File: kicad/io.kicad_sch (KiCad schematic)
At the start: 11 parts, among them J2 UART, P1 Mini-DIN_6pins_ver3, U13 uSD adapter, U14 8259, U16 16550, U17 T6963C

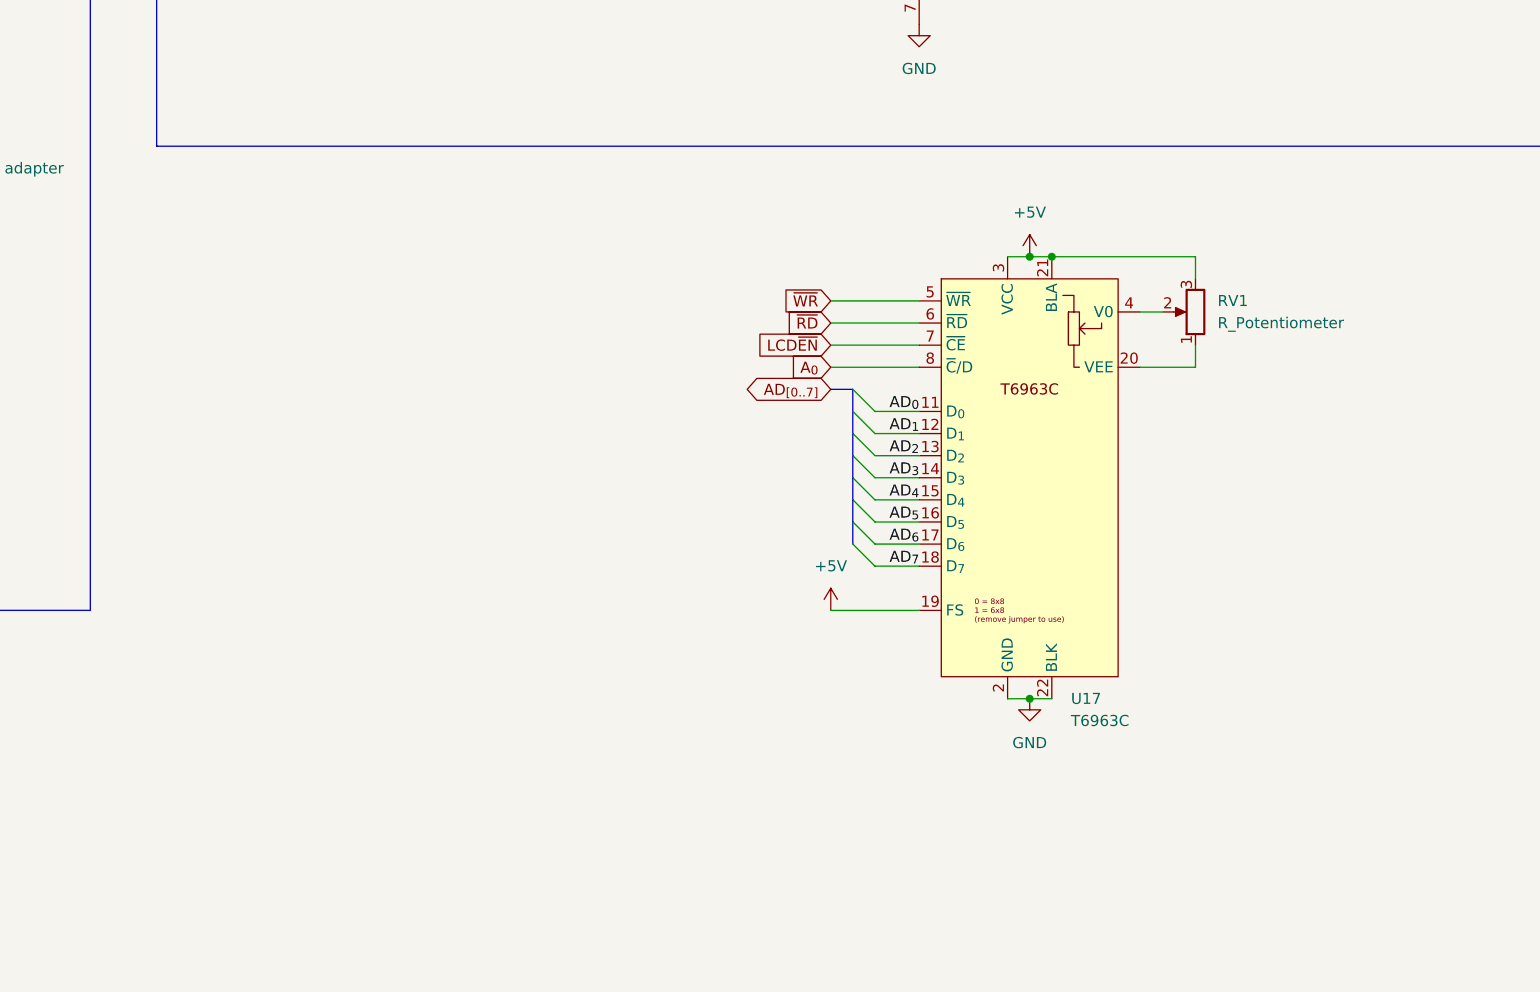
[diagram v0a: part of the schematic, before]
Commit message: Final PCB
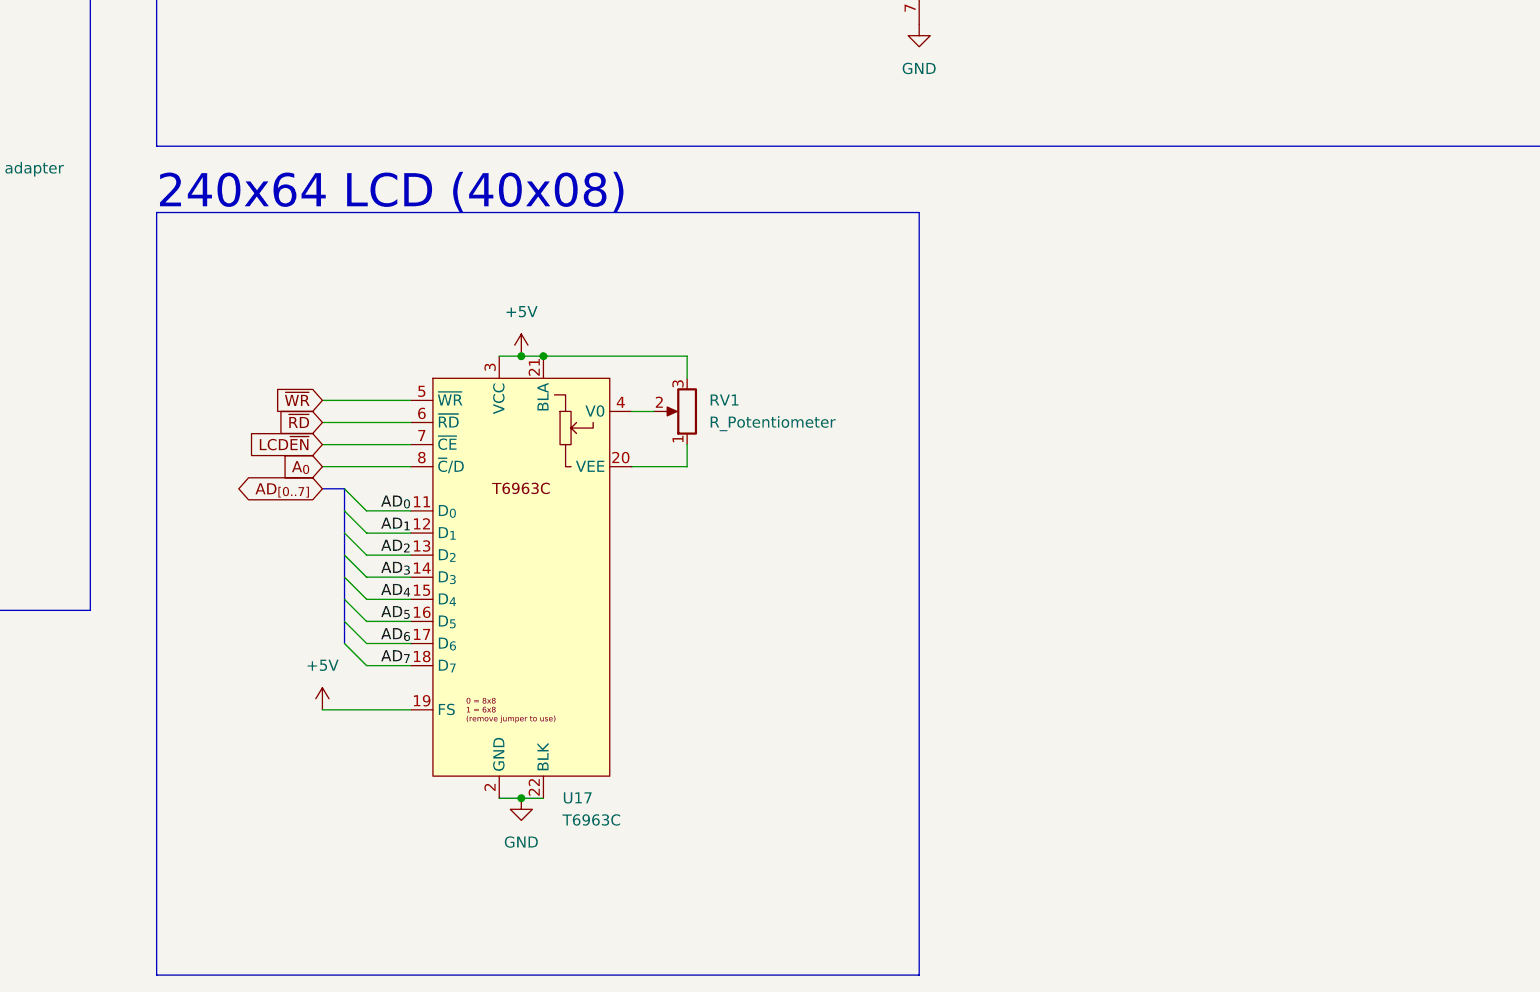
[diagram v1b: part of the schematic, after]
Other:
- note added: "240x64 LCD (40x08)"
- moved on the sheet: RV1, U17
